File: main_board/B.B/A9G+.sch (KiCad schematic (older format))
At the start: 20 parts, among them J7 SIM_Card, J8 Micro_SD_Card, Q13 CJ3134K, Q14 CJ3134K

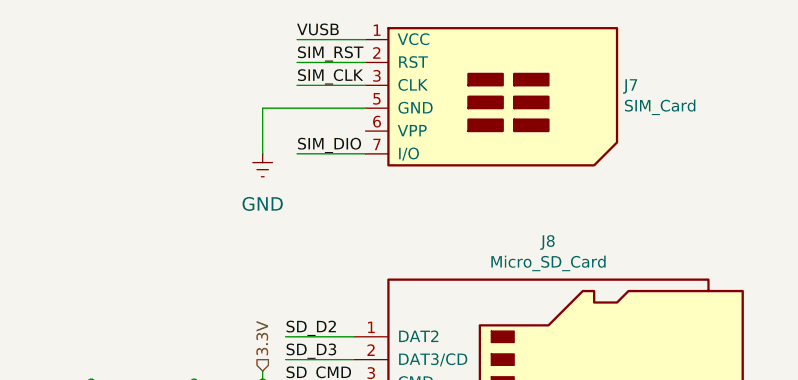
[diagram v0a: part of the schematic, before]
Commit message: start vith pcb
firsxxt proposal component layout of main board
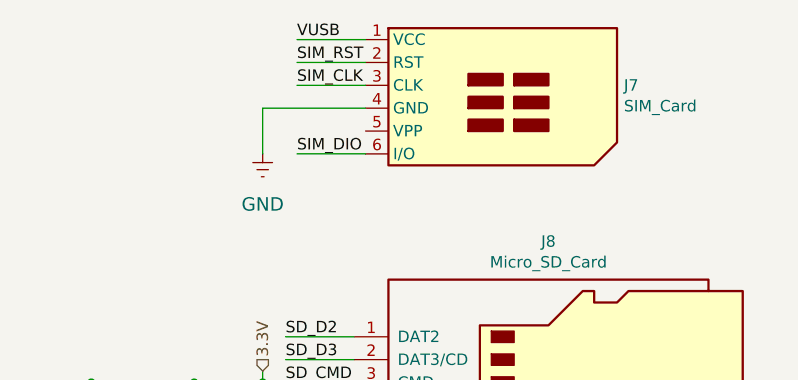
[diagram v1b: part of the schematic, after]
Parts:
- removed J7: SIM_Card, BB:SIM, symbol Connector:SIM_Card
- added J7: SIM_Card, BB:SIM, symbol B.B-rescue:SIM_Card
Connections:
- net SIM_CLK: now also J7.3 (CLK)
- net SIM_DIO: now also J7.6 (I/O)
- net SIM_RST: now also J7.2 (RST)
- net VUSB: now also J7.1 (VCC)
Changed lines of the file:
@@
 EESchema Schematic File Version 4
-LIBS:B.B-cache
-EELAYER 29 0
+EELAYER 30 0
 EELAYER END
 $Descr A4 11693 8268
@@
 F 3 "" H 4000 3800 50  0001 C CNN
 	1    4350 3500
-	1    0    0    -1
-$EndComp
-$Comp
-L Connector:SIM_Card J7
-U 1 1 5F7BD351
-P 9250 1750
-F 0 "J7" H 9880 1850 50  0000 L CNN
-F 1 "SIM_Card" H 9880 1759 50  0000 L CNN
-F 2 "BB:SIM" H 9250 2100 50  0001 C CNN
-F 3 "https://www.we-online.de/katalog/datasheet/693010010601.pdf" H 9200 1750 50  0001 C CNN
-	1    9250 1750
 	1    0    0    -1
 $EndComp
@@
 Connection ~ 8000 2950
 Connection ~ 8000 3350
+$Comp
+L B.B-rescue:SIM_Card J7
+U 1 1 5FAC315F
+P 9250 1750
+F 0 "J7" H 9880 1850 50  0000 L CNN
+F 1 "SIM_Card" H 9880 1759 50  0000 L CNN
+F 2 "BB:SIM" H 9250 2100 50  0001 C CNN
+F 3 "https://www.we-online.de/katalog/datasheet/693010010601.pdf" H 9200 1750 50  0001 C CNN
+	1    9250 1750
+	1    0    0    -1
+$EndComp
 $EndSCHEMATC
